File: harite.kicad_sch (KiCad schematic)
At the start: 10 parts

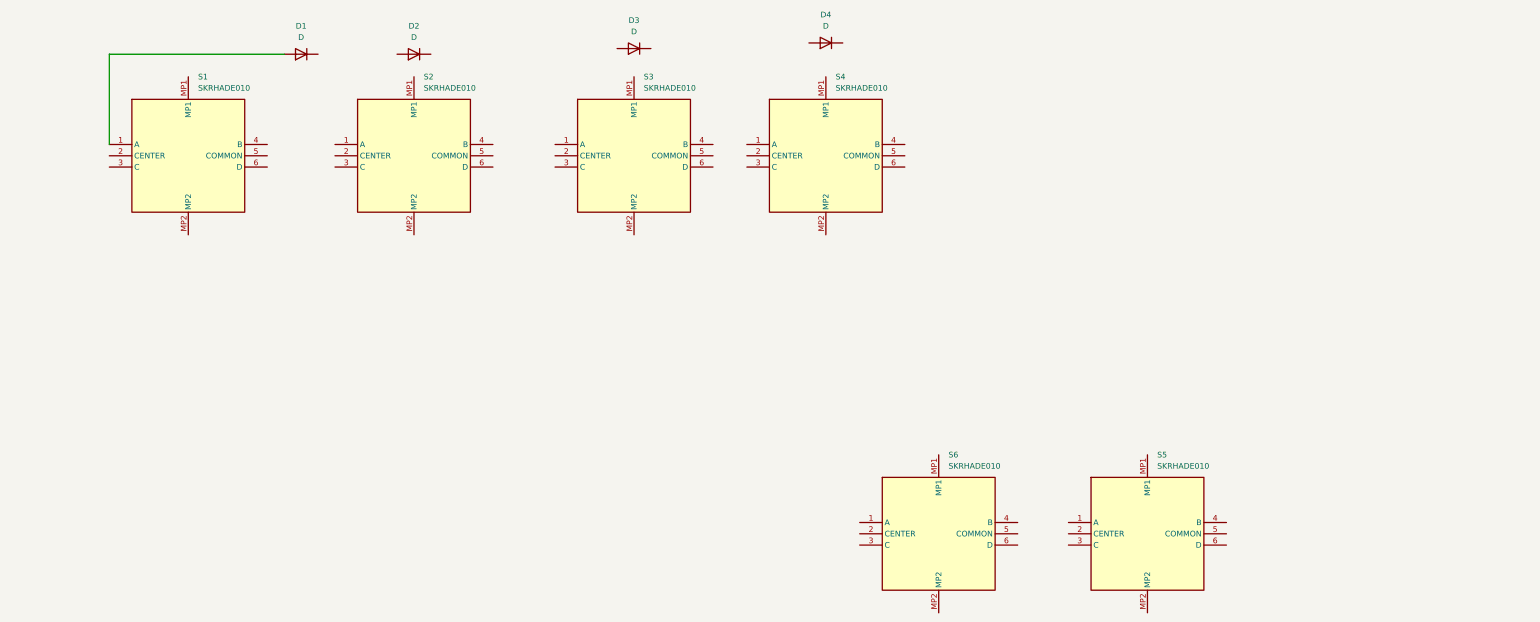
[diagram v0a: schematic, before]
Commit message: Layout switches
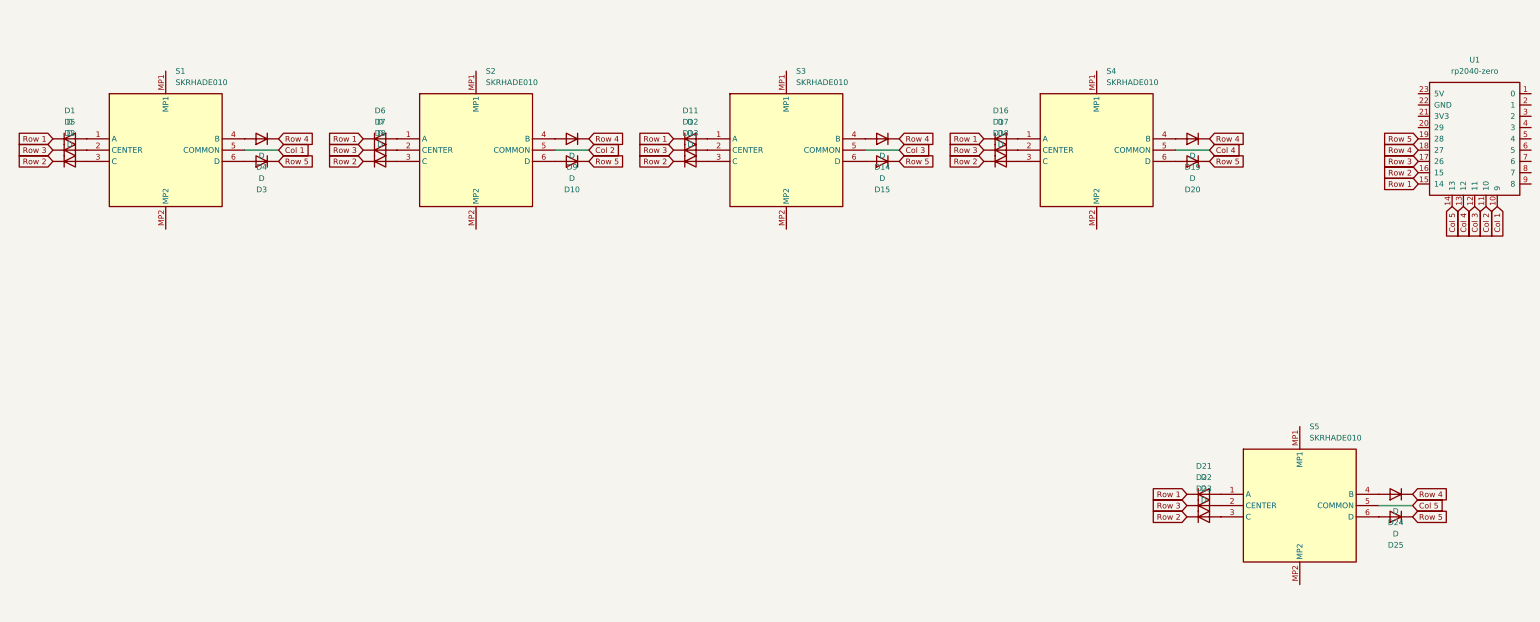
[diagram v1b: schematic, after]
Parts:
- removed S6: SKRHADE010, SKRHADE010, symbol SKRHADE010:SKRHADE010
- added D10, D11, D12, D13, D14, D15, D16, D17, D18, D19, D20, D21, D22, D23, D24, D25, D5, D6, D7, D8, D9: D, footprints:D_SOD123, symbol Device:D
- added U1: rp2040-zero, footprints:rp2040-zero-tht, symbol mcu:rp2040-zero
- D1, D2, D3, D4: footprint (none) -> footprints:D_SOD123
- S1, S2, S3, S4, S5: footprint SKRHADE010 -> footprints:SKRHADE010
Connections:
- net at S1.2 (CENTER): now also D5.2 (A)
- net at S1.3 (C): now also D2.2 (A)
- net at S1.4 (B): now also D4.2 (A)
- net Col 1: now reaches S1.5 (COMMON)
- net Col 1: now also U1.10 (9)
- net at S1.6 (D): now also D3.2 (A)
- net at S3.1 (A): now also D11.2 (A)
- net at S3.2 (CENTER): now also D12.2 (A)
- net at S3.3 (C): now also D13.2 (A)
- net at S3.4 (B): now also D14.2 (A)
- net Col 3: now reaches S3.5 (COMMON)
- net Col 3: now also U1.12 (11)
- net at S3.6 (D): now also D15.2 (A)
- net Row 1: now reaches D1.1 (K)
- net Row 1: now also D11.1 (K), D16.1 (K), D21.1 (K), D6.1 (K), U1.15 (14)
- net at S2.1 (A): now also D6.2 (A)
- net at S2.2 (CENTER): now also D7.2 (A)
- net at S2.3 (C): now also D8.2 (A)
- net at S2.4 (B): now also D9.2 (A)
- net Col 2: now reaches S2.5 (COMMON)
- net Col 2: now also U1.11 (10)
- net at S2.6 (D): now also D10.2 (A)
- net at S4.1 (A): now also D16.2 (A)
- net at S4.2 (CENTER): now also D17.2 (A)
- net at S4.3 (C): now also D18.2 (A)
- net at S4.4 (B): now also D19.2 (A)
- net Col 4: now reaches S4.5 (COMMON)
- net Col 4: now also U1.13 (12)
- net at S4.6 (D): now also D20.2 (A)
- net Row 5: now reaches D3.1 (K)
- net Row 5: now also D10.1 (K), D15.1 (K), D20.1 (K), D25.1 (K), U1.19 (28)
- net Row 4: now reaches D4.1 (K)
- net Row 4: now also D14.1 (K), D19.1 (K), D24.1 (K), D9.1 (K), U1.18 (27)
- net Row 2: now reaches D2.1 (K)
- net Row 2: now also D13.1 (K), D18.1 (K), D23.1 (K), D8.1 (K), U1.16 (15)
- net at S5.1 (A): now also D21.2 (A)
- net at S5.2 (CENTER): now also D22.2 (A)
- net at S5.3 (C): now also D23.2 (A)
- net at S5.4 (B): now also D24.2 (A)
- net Col 5: now reaches S5.5 (COMMON)
- net Col 5: now also U1.14 (13)
- net at S5.6 (D): now also D25.2 (A)
- new net Row 3: D12.1 (K), D17.1 (K), D22.1 (K), D5.1 (K), D7.1 (K), U1.17 (26)
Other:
- moved on the sheet: S1
